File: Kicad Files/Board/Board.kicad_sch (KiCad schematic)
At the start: 35 parts, among them J1 CSP-USC16-TR, SW1 Boot, SW2 RotaryEncoder_Switch, U1 RP2040, U2 W25Q128JVS, U3 USBLC6-2SC6, U4 XC6206PxxxMR, U5 X322512MSB4SI

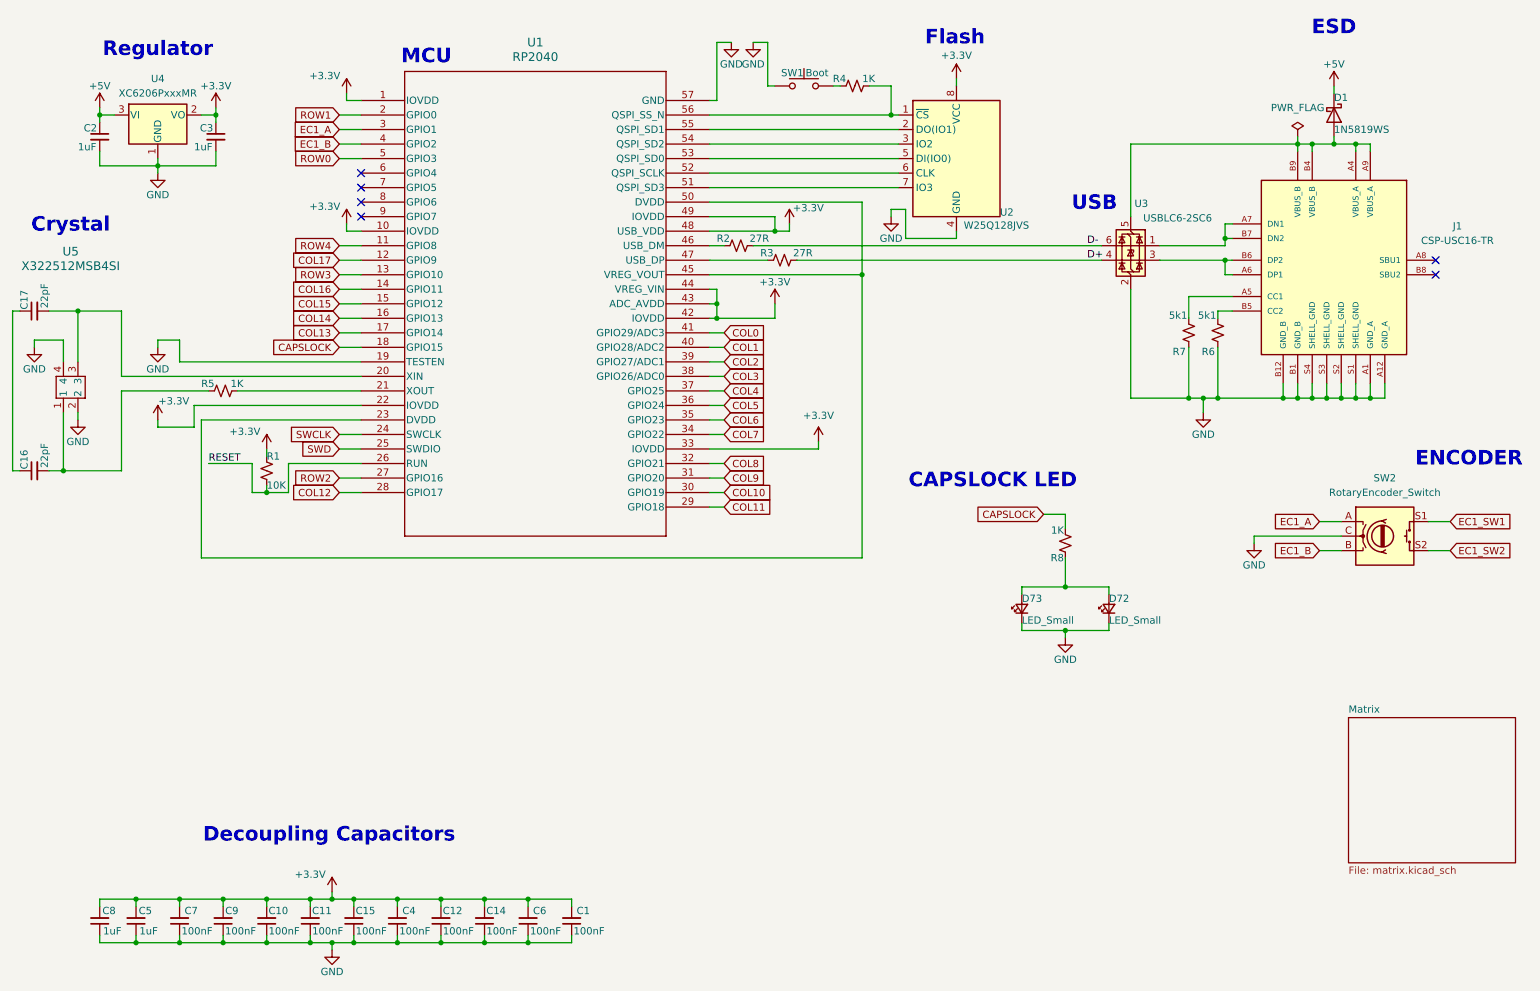
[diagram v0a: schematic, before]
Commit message: PCB Space
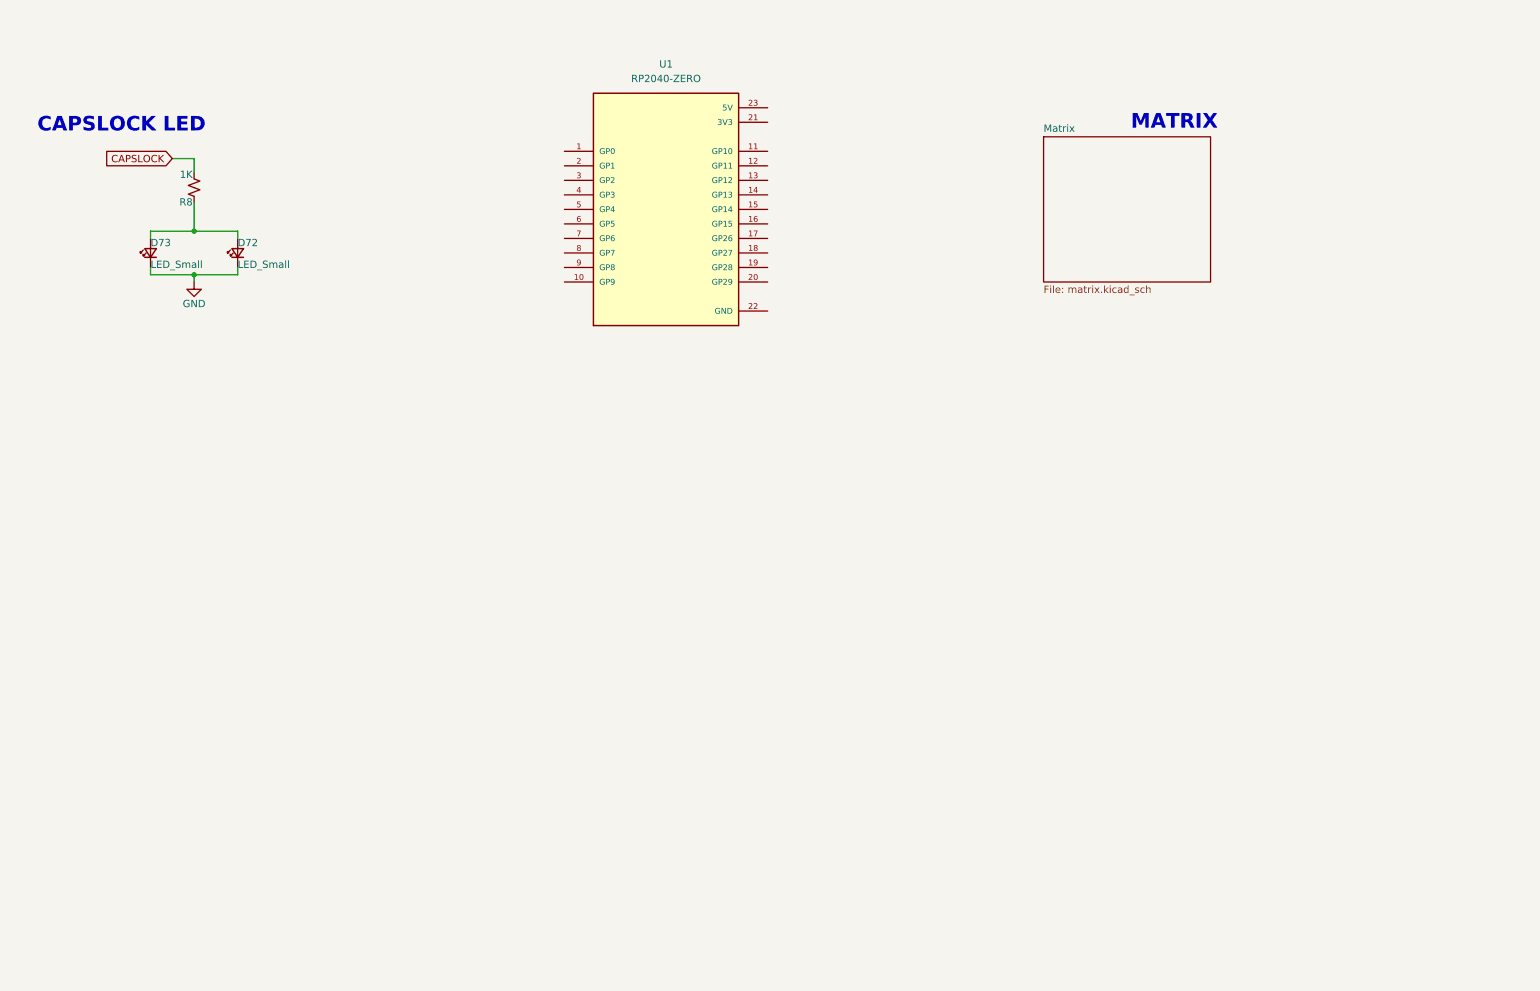
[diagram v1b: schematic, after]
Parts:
- removed C1, C10, C11, C12, C14, C15, C4, C6, C7, C9: 100nF, mechanical_keyboard:C_0402_1005Metric, symbol mechanical_keyboard:C_Small
- removed C16, C17: 22pF, mechanical_keyboard:C_0402_1005Metric, symbol mechanical_keyboard:C_Small
- removed C2, C3, C5, C8: 1uF, mechanical_keyboard:C_0402_1005Metric, symbol mechanical_keyboard:C_Small
- removed D1: 1N5819WS, mechanical_keyboard:D_SOD-323, symbol mechanical_keyboard:1N5819WS
- removed J1: CSP-USC16-TR, mechanical_keyboard:USB_C_Receptacle_HRO_TYPE-C-31-M-12, symbol mechanical_keyboard:CSP-USC16-TR
- removed R1: 10K, mechanical_keyboard:R_0402_1005Metric, symbol Device:R_Small_US
- removed R2, R3: 27R, mechanical_keyboard:R_0402_1005Metric, symbol Device:R_Small_US
- removed R4, R5: 1K, mechanical_keyboard:R_0402_1005Metric, symbol Device:R_Small_US
- removed R6, R7: 5k1, mechanical_keyboard:R_0402_1005Metric, symbol Device:R_Small_US
- removed SW1: Boot, mechanical_keyboard:SW4_KMR221GLFS_CNK, symbol mechanical_keyboard:SW_Push
- removed SW2: RotaryEncoder_Switch, symbol mechanical_keyboard:RotaryEncoder_Switch
- removed U1: RP2040, IC57_RP2040, symbol mechanical_keyboard:RP2040
- removed U2: W25Q128JVS, Package_SO:SOIC-8_5.23x5.23mm_P1.27mm, symbol mechanical_keyboard:W25Q128JVS
- removed U3: USBLC6-2SC6, mechanical_keyboard:SOT-23-6, symbol mechanical_keyboard:USBLC6-2SC6
- removed U4: XC6206PxxxMR, mechanical_keyboard:SOT-23-3, symbol mechanical_keyboard:XC6206PxxxMR
- removed U5: X322512MSB4SI, SMD_2MSB4SI_YXC, symbol mechanical_keyboard:X322512MSB4SI
- added U1: RP2040-ZERO, mechanical_keyboard:MODULE_RP2040-ZERO, symbol mechanical_keyboard:RP2040-ZERO
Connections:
- no-connect marks 6 -> 0
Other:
- note added: "MATRIX"
- note removed: "Crystal"
- note removed: "Decoupling Capacitors"
- note removed: "ENCODER"
- note removed: "ESD"
- note removed: "Flash"
- note removed: "MCU"
- note removed: "Regulator"
- note removed: "USB"
- moved on the sheet: D72, D73, R8

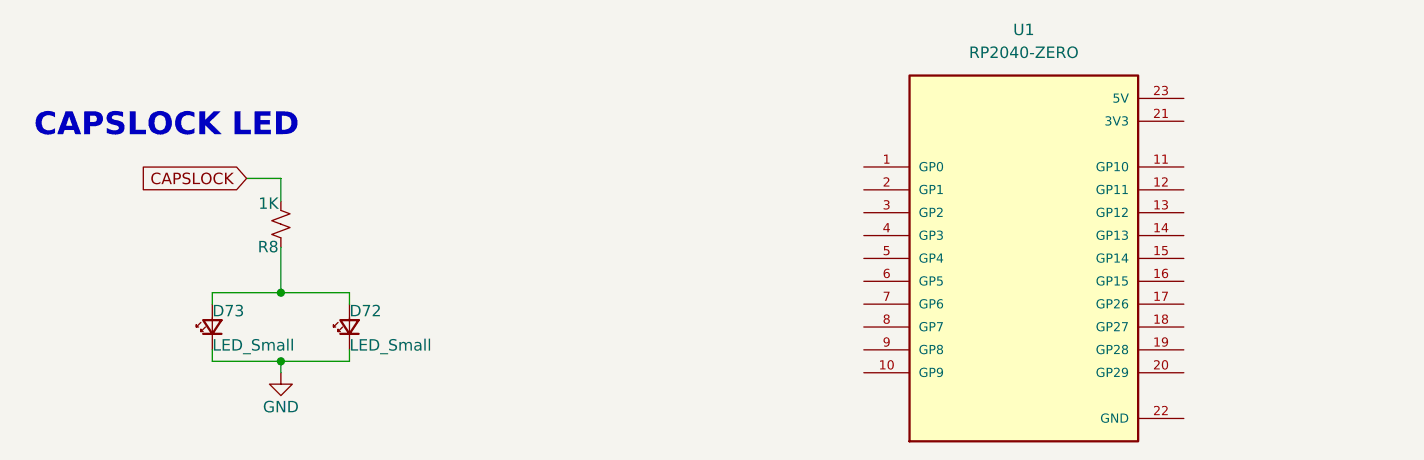
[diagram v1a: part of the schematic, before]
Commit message: Routing Completed
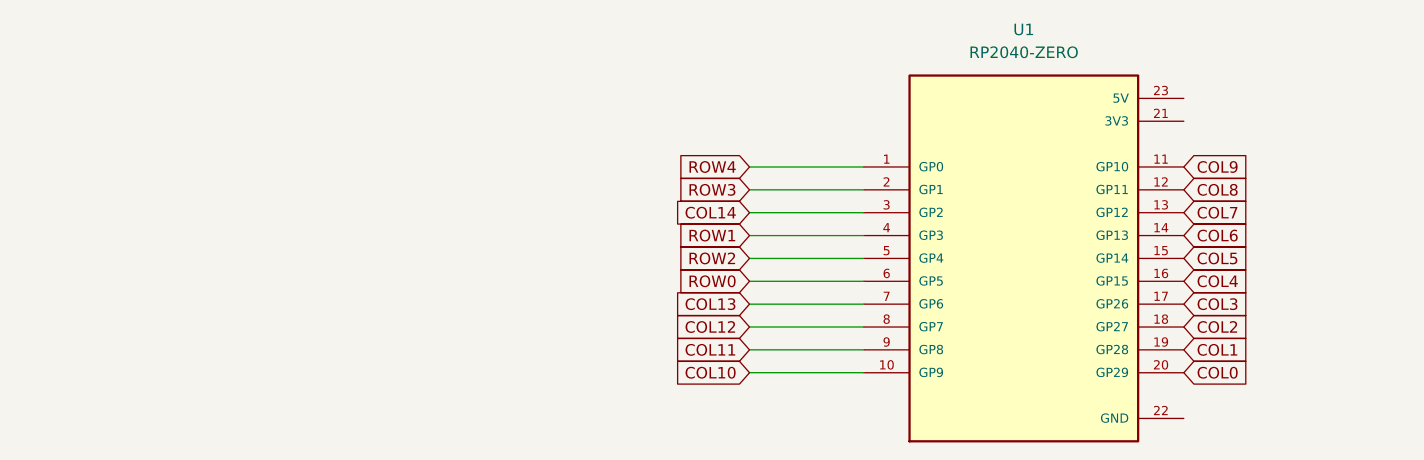
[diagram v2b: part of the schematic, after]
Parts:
- removed D72, D73: LED_Small, mechanical_keyboard:LED_0603_1608Metric, symbol mechanical_keyboard:LED_Small
- removed R8: 1K, mechanical_keyboard:R_0402_1005Metric, symbol Device:R_Small_US
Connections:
- net ROW4: now reaches U1.1 (GP0)
- net COL10: now reaches U1.10 (GP9)
- net COL9: now reaches U1.11 (GP10)
- net COL8: now reaches U1.12 (GP11)
- net COL7: now reaches U1.13 (GP12)
- net COL6: now reaches U1.14 (GP13)
- net COL5: now reaches U1.15 (GP14)
- net COL4: now reaches U1.16 (GP15)
- net COL3: now reaches U1.17 (GP26)
- net COL2: now reaches U1.18 (GP27)
- net COL1: now reaches U1.19 (GP28)
- net ROW3: now reaches U1.2 (GP1)
- net COL0: now reaches U1.20 (GP29)
- net COL14: now reaches U1.3 (GP2)
- net ROW1: now reaches U1.4 (GP3)
- net ROW2: now reaches U1.5 (GP4)
- net ROW0: now reaches U1.6 (GP5)
- net COL13: now reaches U1.7 (GP6)
- net COL12: now reaches U1.8 (GP7)
- net COL11: now reaches U1.9 (GP8)
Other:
- note removed: "CAPSLOCK LED"
